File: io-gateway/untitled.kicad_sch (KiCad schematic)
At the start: 8 parts, among them J1 1752201, J2 1752201, J3 1752201, J4 Screw_Terminal_01x09, J5 Screw_Terminal_01x09, J6 Screw_Terminal_01x09

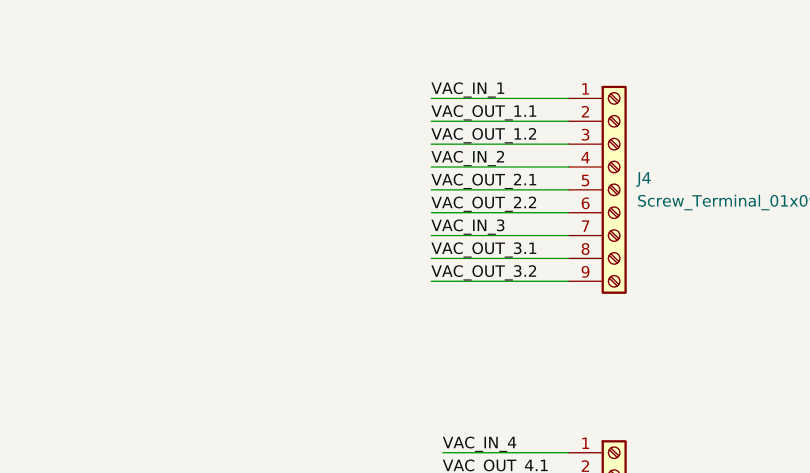
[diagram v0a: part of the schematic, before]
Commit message: add relays
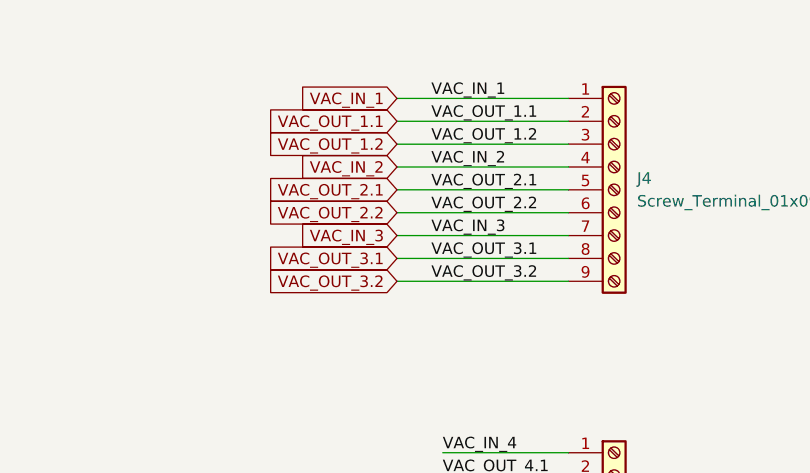
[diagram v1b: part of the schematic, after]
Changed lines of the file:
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@@
-	(wire
-		(pts
-			(xy 238.76 27.94) (xy 254 27.94)
-		)
-		(stroke
-			(width 0)
-			(type default)
-		)
-	)
 	(wire
 		(pts
@@
 	(wire
 		(pts
-			(xy 238.76 38.1) (xy 254 38.1)
+			(xy 234.95 30.48) (xy 254 30.48)
 		)
 		(stroke
@@
 	(wire
 		(pts
+			(xy 234.95 33.02) (xy 254 33.02)
+		)
+		(stroke
+			(width 0)
+			(type default)
+		)
+	)
+	(wire
+		(pts
 			(xy 40.64 39.37) (xy 44.45 39.37)
 		)
@@
 	(wire
 		(pts
+			(xy 234.95 40.64) (xy 254 40.64)
+		)
+		(stroke
+			(width 0)
+			(type default)
+		)
+	)
+	(wire
+		(pts
+			(xy 234.95 27.94) (xy 254 27.94)
+		)
+		(stroke
+			(width 0)
+			(type default)
+		)
+	)
+	(wire
+		(pts
 			(xy 41.91 142.24) (xy 45.72 142.24)
 		)
@@
 	(wire
 		(pts
-			(xy 238.76 40.64) (xy 254 40.64)
-		)
-		(stroke
-			(width 0)
-			(type default)
-		)
-	)
-	(wire
-		(pts
 			(xy 40.64 44.45) (xy 44.45 44.45)
 		)
@@
 	(wire
 		(pts
-			(xy 238.76 35.56) (xy 254 35.56)
-		)
-		(stroke
-			(width 0)
-			(type default)
-		)
-	)
-	(wire
-		(pts
 			(xy 40.64 95.25) (xy 45.72 95.25)
 		)
@@
 	(wire
 		(pts
-			(xy 238.76 45.72) (xy 254 45.72)
-		)
-		(stroke
-			(width 0)
-			(type default)
-		)
-	)
-	(wire
-		(pts
 			(xy 240.03 118.11) (xy 252.73 118.11)
 		)
@@
 	(wire
 		(pts
+			(xy 234.95 45.72) (xy 254 45.72)
+		)
+		(stroke
+			(width 0)
+			(type default)
+		)
+	)
+	(wire
+		(pts
 			(xy 41.91 162.56) (xy 45.72 162.56)
 		)
@@
 	(wire
 		(pts
+			(xy 234.95 25.4) (xy 254 25.4)
+		)
+		(stroke
+			(width 0)
+			(type default)
+		)
+	)
+	(wire
+		(pts
 			(xy 240.03 69.85) (xy 254 69.85)
 		)
@@
 	(wire
 		(pts
+			(xy 234.95 38.1) (xy 254 38.1)
+		)
+		(stroke
+			(width 0)
+			(type default)
+		)
+	)
+	(wire
+		(pts
+			(xy 234.95 43.18) (xy 254 43.18)
+		)
+		(stroke
+			(width 0)
+			(type default)
+		)
+	)
+	(wire
+		(pts
 			(xy 240.03 74.93) (xy 254 74.93)
 		)
@@
 	(wire
 		(pts
-			(xy 238.76 25.4) (xy 254 25.4)
-		)
-		(stroke
-			(width 0)
-			(type default)
-		)
-	)
-	(wire
-		(pts
 			(xy 240.03 120.65) (xy 252.73 120.65)
 		)
@@
 	(wire
 		(pts
+			(xy 234.95 35.56) (xy 254 35.56)
+		)
+		(stroke
+			(width 0)
+			(type default)
+		)
+	)
+	(wire
+		(pts
 			(xy 40.64 29.21) (xy 44.45 29.21)
 		)
@@
 	(wire
 		(pts
-			(xy 238.76 30.48) (xy 254 30.48)
-		)
-		(stroke
-			(width 0)
-			(type default)
-		)
-	)
-	(wire
-		(pts
-			(xy 238.76 43.18) (xy 254 43.18)
-		)
-		(stroke
-			(width 0)
-			(type default)
-		)
-	)
-	(wire
-		(pts
 			(xy 123.19 26.67) (xy 114.3 26.67)
 		)
@@
 		(pts
 			(xy 41.91 152.4) (xy 45.72 152.4)
-		)
-		(stroke
-			(width 0)
-			(type default)
-		)
-	)
-	(wire
-		(pts
-			(xy 238.76 33.02) (xy 254 33.02)
 		)
 		(stroke
@@
 		)
 	)
+	(global_label "VAC_OUT_2.2"
+		(shape input)
+		(at 234.95 38.1 180)
+		(fields_autoplaced yes)
+		(effects
+			(font
+				(size 1.27 1.27)
+			)
+			(justify right)
+		)
+		(property "Intersheetrefs" "${INTERSHEET_REFS}"
+			(at 219.93 38.1 0)
+			(effects
+				(font
+					(size 1.27 1.27)
+				)
+				(justify right)
+				(hide yes)
+			)
+		)
+	)
+	(global_label "VAC_OUT_3.1"
+		(shape input)
+		(at 234.95 43.18 180)
+		(fields_autoplaced yes)
+		(effects
+			(font
+				(size 1.27 1.27)
+			)
+			(justify right)
+		)
+		(property "Intersheetrefs" "${INTERSHEET_REFS}"
+			(at 219.93 43.18 0)
+			(effects
+				(font
+					(size 1.27 1.27)
+				)
+				(justify right)
+				(hide yes)
+			)
+		)
+	)
+	(global_label "VAC_IN_2"
+		(shape input)
+		(at 234.95 33.02 180)
+		(fields_autoplaced yes)
+		(effects
+			(font
+				(size 1.27 1.27)
+			)
+			(justify right)
+		)
+		(property "Intersheetrefs" "${INTERSHEET_REFS}"
+			(at 223.4376 33.02 0)
+			(effects
+				(font
+					(size 1.27 1.27)
+				)
+				(justify right)
+				(hide yes)
+			)
+		)
+	)
+	(global_label "VAC_OUT_3.2"
+		(shape input)
+		(at 234.95 45.72 180)
+		(fields_autoplaced yes)
+		(effects
+			(font
+				(size 1.27 1.27)
+			)
+			(justify right)
+		)
+		(property "Intersheetrefs" "${INTERSHEET_REFS}"
+			(at 219.93 45.72 0)
+			(effects
+				(font
+					(size 1.27 1.27)
+				)
+				(justify right)
+				(hide yes)
+			)
+		)
+	)
+	(global_label "VAC_OUT_2.1"
+		(shape input)
+		(at 234.95 35.56 180)
+		(fields_autoplaced yes)
+		(effects
+			(font
+				(size 1.27 1.27)
+			)
+			(justify right)
+		)
+		(property "Intersheetrefs" "${INTERSHEET_REFS}"
+			(at 219.93 35.56 0)
+			(effects
+				(font
+					(size 1.27 1.27)
+				)
+				(justify right)
+				(hide yes)
+			)
+		)
+	)
+	(global_label "VAC_IN_3"
+		(shape input)
+		(at 234.95 40.64 180)
+		(fields_autoplaced yes)
+		(effects
+			(font
+				(size 1.27 1.27)
+			)
+			(justify right)
+		)
+		(property "Intersheetrefs" "${INTERSHEET_REFS}"
+			(at 223.4376 40.64 0)
+			(effects
+				(font
+					(size 1.27 1.27)
+				)
+				(justify right)
+				(hide yes)
+			)
+		)
+	)
+	(global_label "VAC_OUT_1.2"
+		(shape input)
+		(at 234.95 30.48 180)
+		(fields_autoplaced yes)
+		(effects
+			(font
+				(size 1.27 1.27)
+			)
+			(justify right)
+		)
+		(property "Intersheetrefs" "${INTERSHEET_REFS}"
+			(at 219.93 30.48 0)
+			(effects
+				(font
+					(size 1.27 1.27)
+				)
+				(justify right)
+				(hide yes)
+			)
+		)
+	)
+	(global_label "VAC_OUT_1.1"
+		(shape input)
+		(at 234.95 27.94 180)
+		(fields_autoplaced yes)
+		(effects
+			(font
+				(size 1.27 1.27)
+			)
+			(justify right)
+		)
+		(property "Intersheetrefs" "${INTERSHEET_REFS}"
+			(at 219.93 27.94 0)
+			(effects
+				(font
+					(size 1.27 1.27)
+				)
+				(justify right)
+				(hide yes)
+			)
+		)
+	)
+	(global_label "VAC_IN_1"
+		(shape input)
+		(at 234.95 25.4 180)
+		(fields_autoplaced yes)
+		(effects
+			(font
+				(size 1.27 1.27)
+			)
+			(justify right)
+		)
+		(property "Intersheetrefs" "${INTERSHEET_REFS}"
+			(at 223.4376 25.4 0)
+			(effects
+				(font
+					(size 1.27 1.27)
+				)
+				(justify right)
+				(hide yes)
+			)
+		)
+	)
